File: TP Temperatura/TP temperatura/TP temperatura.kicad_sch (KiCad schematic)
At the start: 12 parts, among them SW1 SW_Push, SW2 SW_Push, U1 D198K, U2 D198K, U3 74HC595

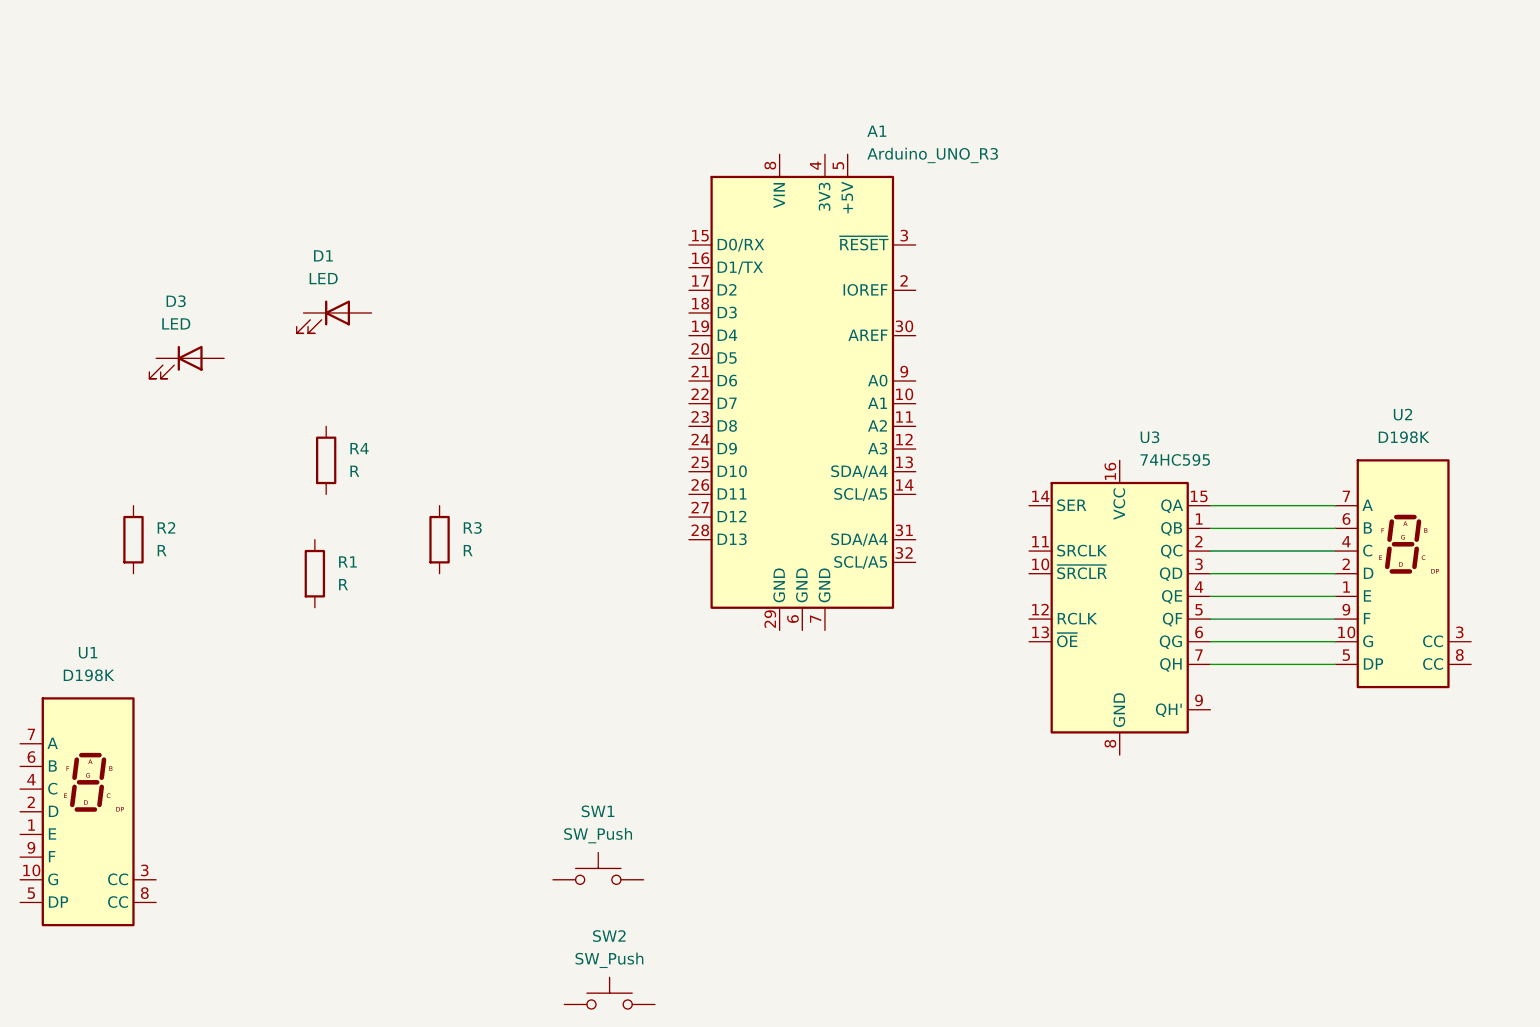
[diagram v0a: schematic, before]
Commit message: TP Temperatura
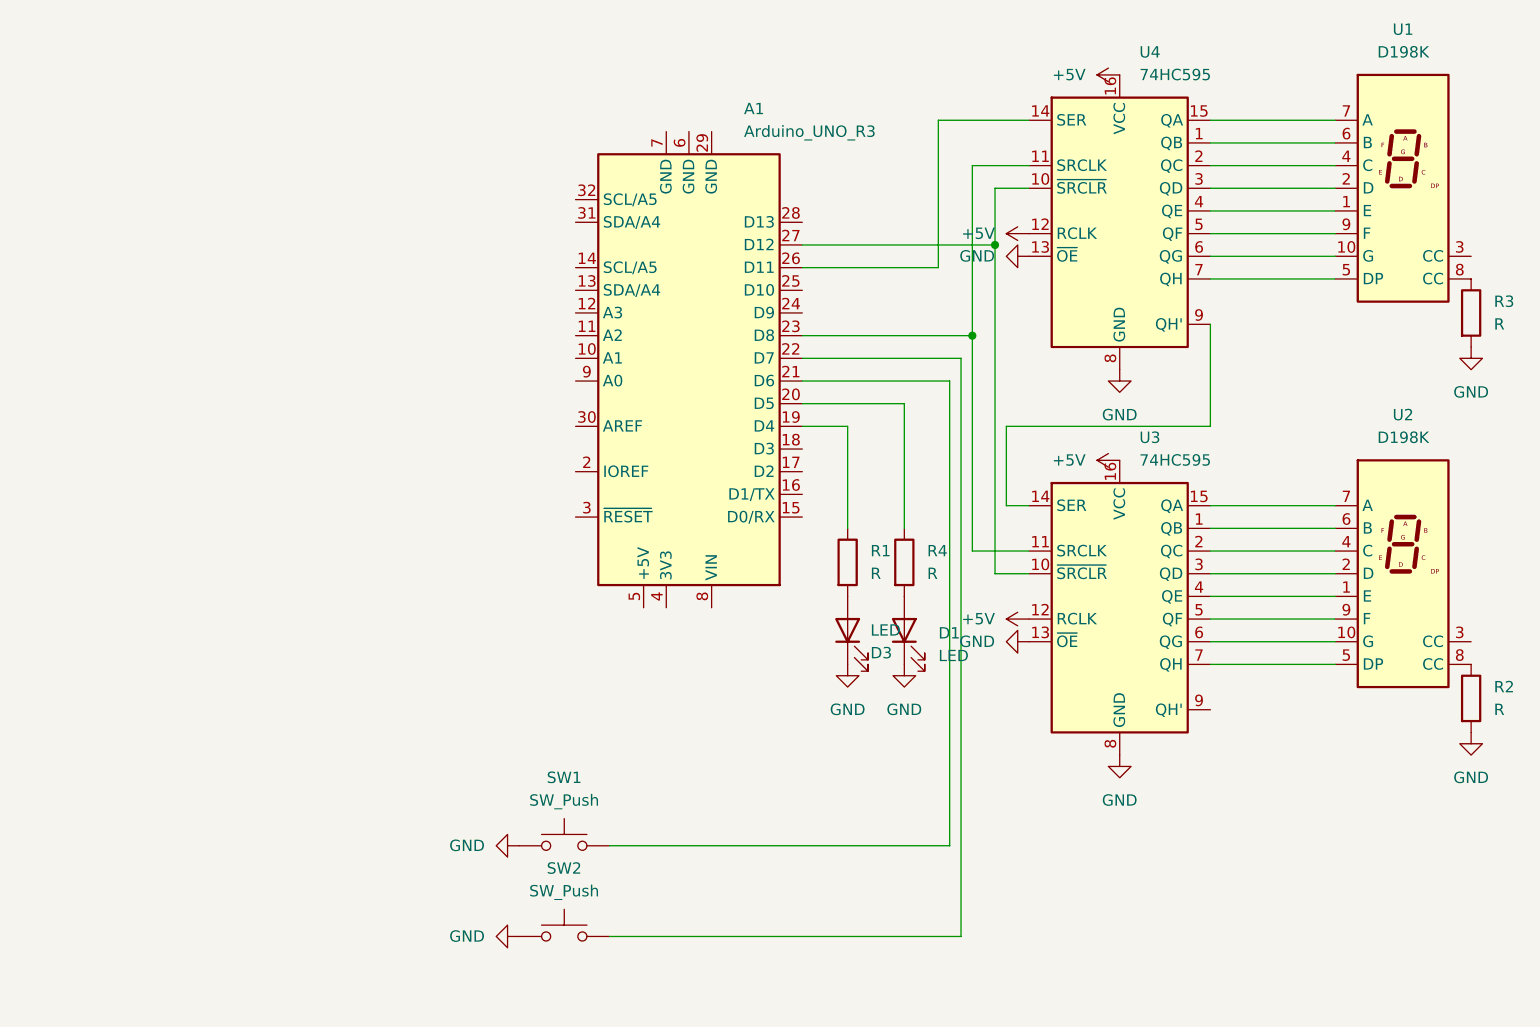
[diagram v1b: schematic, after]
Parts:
- added U4: 74HC595, Package_DIP:DIP-16_W7.62mm_LongPads, symbol 74xx:74HC595
- SW1, SW2: footprint (none) -> Button_Switch_THT:SW_PUSH_6mm
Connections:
- net at R1.1: now also A1.19 (D4)
- net at R1.2: now also D3.2 (A)
- net at R4.1: now also A1.20 (D5)
- net at R4.2: now also D1.2 (A)
- net at A1.21 (D6): now also SW1.2
- net at A1.22 (D7): now also SW2.2
- net at A1.23 (D8): now also U3.11 (SRCLK), U4.11 (SRCLK)
- net at A1.26 (D11): now also U4.14 (SER)
- net at A1.27 (D12): now also U3.10 (~{SRCLR}), U4.10 (~{SRCLR})
- net at R2.1: now also U2.8 (CC)
- net GND: now reaches R2.2
- net GND: now also D1.1 (K), D3.1 (K), R3.2, SW1.1, SW2.1, U3.13 (~{OE}), U3.8 (GND), U4.13 (~{OE}), U4.8 (GND)
- net at R3.1: now also U1.8 (CC)
- net +5V: now reaches U3.12 (RCLK)
- net +5V: now also U3.16 (VCC), U4.12 (RCLK), U4.16 (VCC)
- net at U3.14 (SER): now also U4.9 (QH')
- net at U1.1 (E): now also U4.4 (QE)
- net at U1.10 (G): now also U4.6 (QG)
- net at U1.2 (D): now also U4.3 (QD)
- net at U1.4 (C): now also U4.2 (QC)
- net at U1.5 (DP): now also U4.7 (QH)
- net at U1.6 (B): now also U4.1 (QB)
- net at U1.7 (A): now also U4.15 (QA)
- net at U1.9 (F): now also U4.5 (QF)
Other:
- moved on the sheet: A1, D1, D3, R1, R4, SW1
